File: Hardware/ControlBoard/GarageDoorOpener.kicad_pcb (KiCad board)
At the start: 2 copper layers, 70 x 55 mm, 48 parts, among them J1 Conn_01x04, J2 RJ45, Q1 DMG1012T-7, U1 Argon/Boron, U2 TPS56637, U3 CPC1002N, U4 VL53L1X

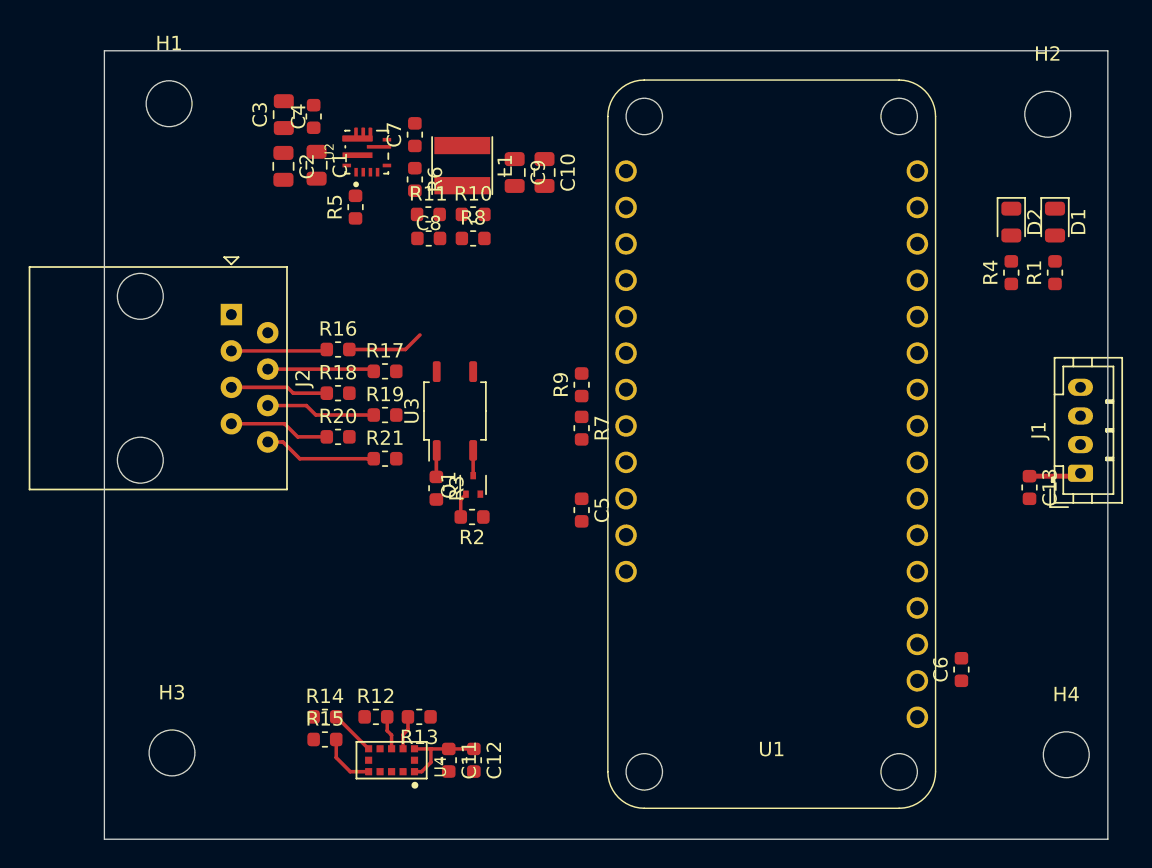
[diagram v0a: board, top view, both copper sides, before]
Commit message: first pass of completed control board done
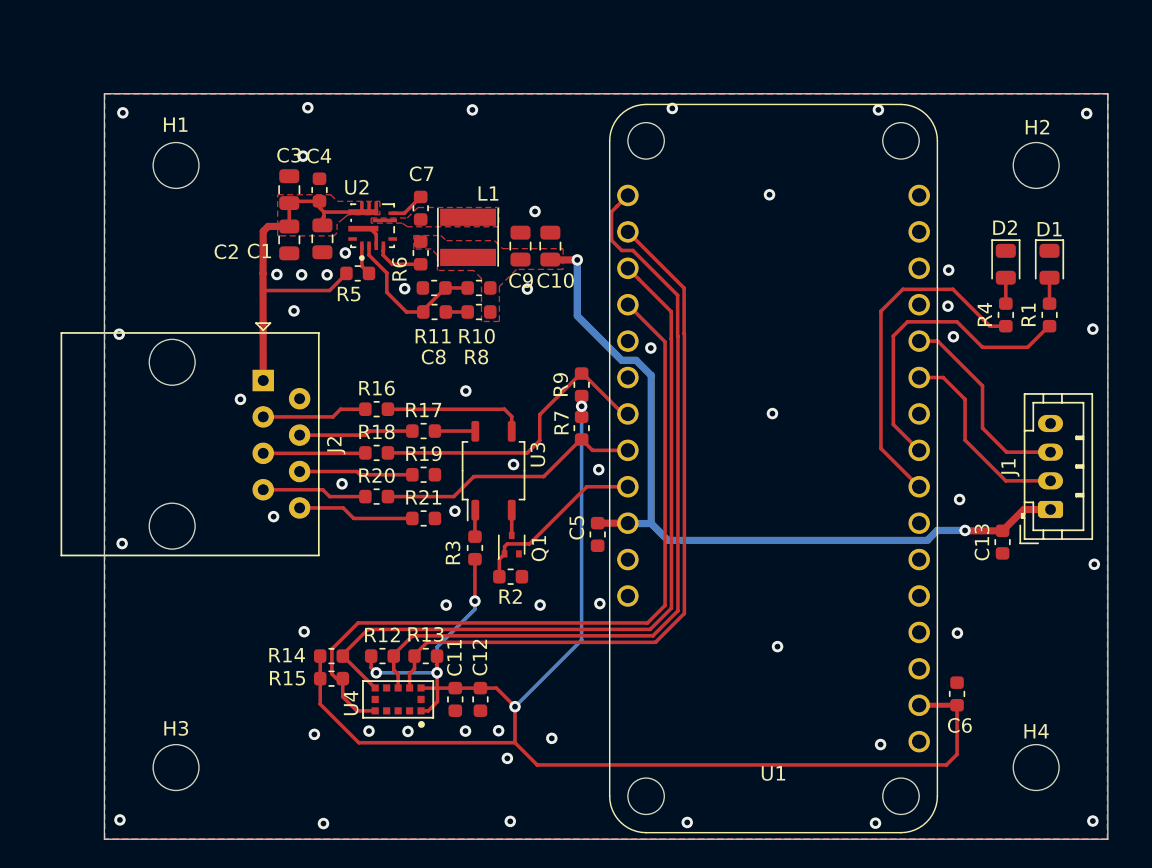
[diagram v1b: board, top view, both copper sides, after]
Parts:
- moved C3 5.25 mm to (110.9, 74.1)
- moved C1 5.15 mm to (113.2, 77.5)
- moved C2 5.15 mm to (110.9, 77.6)
- moved C8 5.15 mm to (121.0, 82.6)
- moved R10 5.15 mm to (124.1, 80.9)
- moved R11 5.15 mm to (121.0, 80.9)
- moved R8 5.15 mm to (124.1, 82.6)
- moved C4 5.15 mm to (113.0, 74.1)
- moved C7 5.15 mm to (120.1, 75.4)
- moved R6 5.15 mm to (120.1, 78.5)
- moved U2 5.15 mm to (116.7, 76.6)
- moved C10 5.15 mm to (129.1, 78.0)
- moved C9 5.15 mm to (127.0, 78.0)
- moved J2 5.11 mm to (109.1, 87.4)
- moved L1 5.02 mm to (123.4, 77.4)
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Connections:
- R19 pad 2: /REED_SW2_GND -> GND
- R21 pad 2: /REED_SW1_GND -> GND
- R7 pad 2: /REED_SW1 -> /REED_SW1_IN
- R9 pad 2: /REED_SW2 -> /REED_SW2_IN
- U1 pad 23: /REED_SW2 -> /REED_SW2_IN
- U1 pad 24: /REED_SW1 -> /REED_SW1_IN
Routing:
- net +3V3: track 6.50 -> 109.1 mm, vias 0 -> 5
- net /SENSOR_I2C_SDA: track 2.35 -> 55.4 mm
- net +5V: track 3.64 -> 56.0 mm, vias 0 -> 2
- net /SENSOR_INT: track 3.18 -> 52.5 mm
- net /SENSOR_SHUTDOWN: track 3.94 -> 53.1 mm
- net /SENSOR_I2C_SCL: track 2.36 -> 50.7 mm
- net +24V: track 0.00 -> 28.3 mm
- net /STATUS_LED: track 0.00 -> 23.8 mm
- net /CONNECTIVITY_LED: track 0.00 -> 21.4 mm
- net /REED_SW2_IN: track 0.00 -> 21.3 mm
- net /REED_SW1_IN: track 0.00 -> 18.7 mm
- net /LED_STRIP_DATA: track 0.00 -> 14.1 mm
- net /LED_STRIP_CLK: track 0.00 -> 13.8 mm
- net /RELAY_CTRL1: track 1.74 -> 12.6 mm
- net Net-(C8-Pad1): track 0.00 -> 10.7 mm
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- added copper zone on F.Cu, net +24V
- added copper zone on F.Cu, net +5V
- added copper zone on B.Cu, net GND
- added copper zone on F.Cu, net GND
- added copper zone on F.Cu, net Net-(C7-Pad1)
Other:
- board size 70 x 55 mm -> 70 x 52 mm
